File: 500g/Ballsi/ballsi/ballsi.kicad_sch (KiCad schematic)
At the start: 4 parts, among them J1 Conn_01x03, J2 Conn_01x03, J3 Conn_01x03

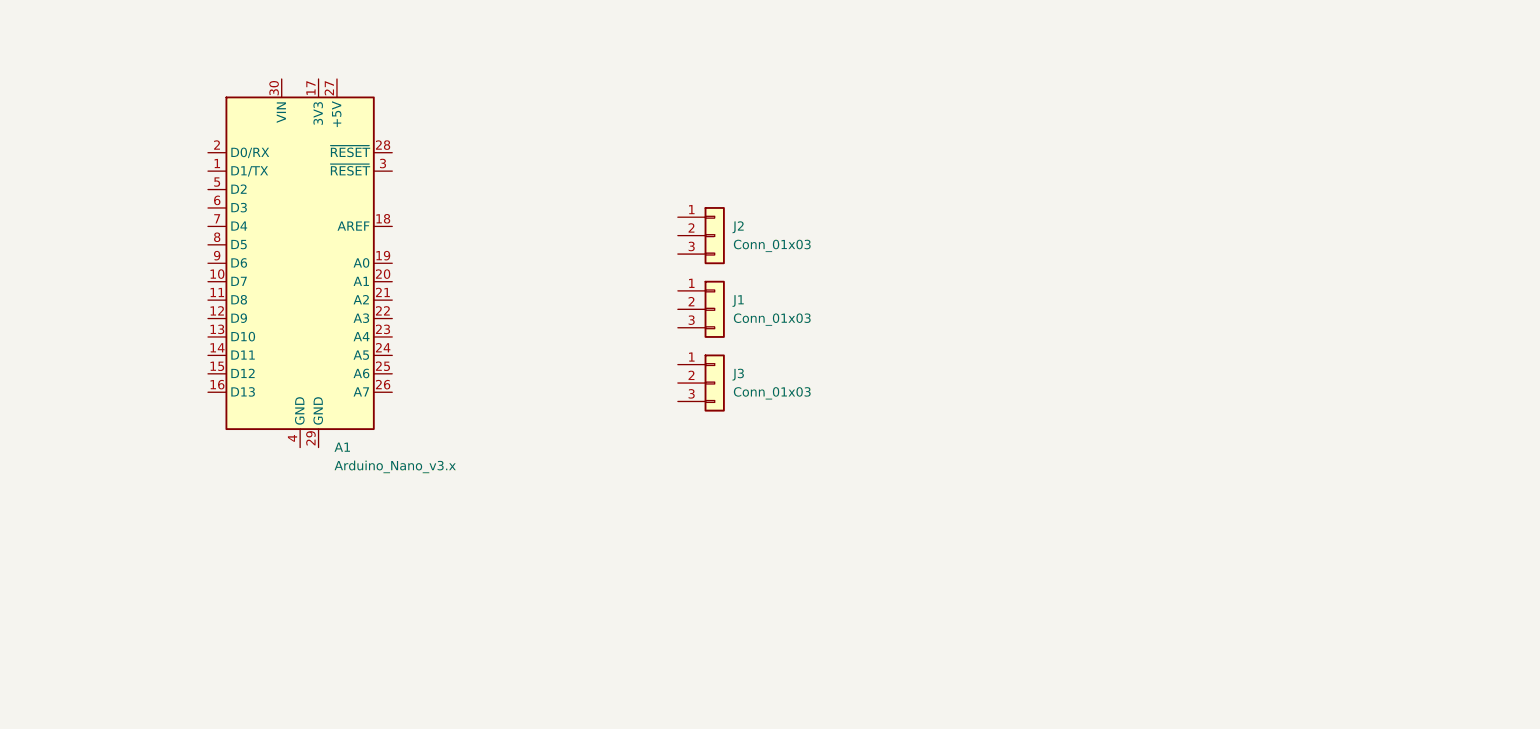
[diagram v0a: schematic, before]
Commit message: added microcontroller sensors and motordriver
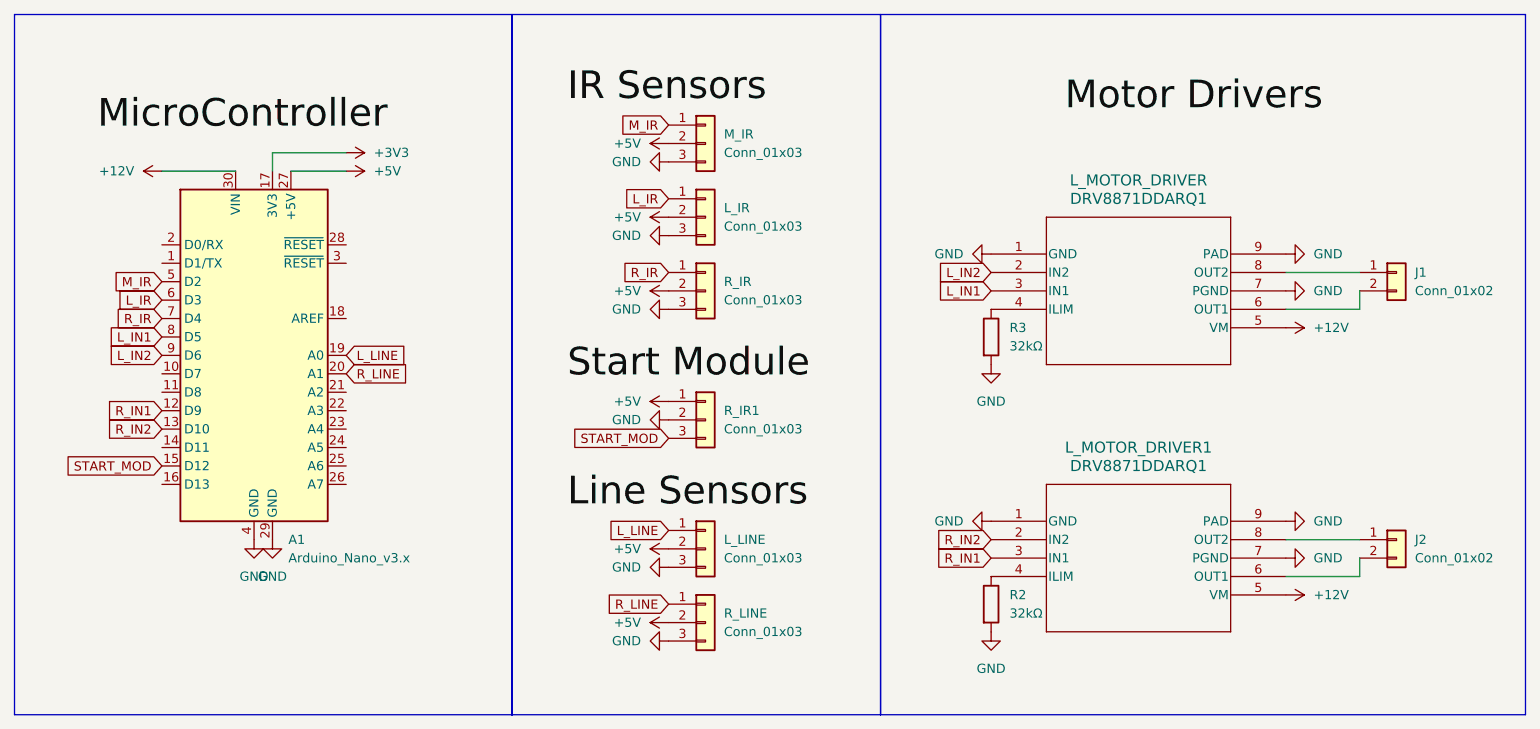
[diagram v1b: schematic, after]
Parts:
- added J1, J2: Conn_01x02, symbol Connector_Generic:Conn_01x02
- added L_LINE, R_IR1, R_LINE: Conn_01x03, Connector_JST:JST_PH_B3B-PH-K_1x03_P2.00mm_Vertical, symbol Connector_Generic:Conn_01x03
- added L_MOTOR_DRIVER, L_MOTOR_DRIVER1: DRV8871DDARQ1, DDA0008H_N_TEX, symbol DRV8871:DRV8871DDARQ1
- added R2, R3: 32kΩ, symbol Device:R
- renumbered J1 to L_IR, J2 to M_IR, J3 to R_IR
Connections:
- net R_IN1: now reaches A1.12 (D9)
- net R_IN1: now also L_MOTOR_DRIVER1.3 (IN1)
- net R_IN2: now reaches A1.13 (D10)
- net R_IN2: now also L_MOTOR_DRIVER1.2 (IN2)
- net START_MOD: now reaches A1.15 (D12)
- net START_MOD: now also R_IR1.3 (Pin_3)
- net +3V3: now reaches A1.17 (3V3)
- net L_LINE: now reaches A1.19 (A0)
- net L_LINE: now also L_LINE.1 (Pin_1)
- net R_LINE: now reaches A1.20 (A1)
- net R_LINE: now also R_LINE.1 (Pin_1)
- net +5V: now reaches A1.27 (+5V)
- net +5V: now also L_IR.2 (Pin_2), M_IR.2 (Pin_2), R_IR.2 (Pin_2), L_LINE.2 (Pin_2), R_IR1.1 (Pin_1), R_LINE.2 (Pin_2)
- net GND: now reaches A1.29 (GND)
- net GND: now also A1.4 (GND), L_IR.3 (Pin_3), M_IR.3 (Pin_3), R_IR.3 (Pin_3), L_LINE.3 (Pin_3), L_MOTOR_DRIVER.1 (GND), L_MOTOR_DRIVER.7 (PGND), L_MOTOR_DRIVER.9 (PAD), L_MOTOR_DRIVER1.1 (GND), L_MOTOR_DRIVER1.7 (PGND), L_MOTOR_DRIVER1.9 (PAD), R2.2, R3.2, R_IR1.2 (Pin_2), R_LINE.3 (Pin_3)
- net +12V: now reaches A1.30 (VIN)
- net +12V: now also L_MOTOR_DRIVER.5 (VM), L_MOTOR_DRIVER1.5 (VM)
- net M_IR: now reaches A1.5 (D2)
- net M_IR: now also M_IR.1 (Pin_1)
- net L_IR: now reaches A1.6 (D3)
- net L_IR: now also L_IR.1 (Pin_1)
- net R_IR: now reaches A1.7 (D4)
- net R_IR: now also R_IR.1 (Pin_1)
- net L_IN1: now reaches A1.8 (D5)
- net L_IN1: now also L_MOTOR_DRIVER.3 (IN1)
- net L_IN2: now reaches A1.9 (D6)
- net L_IN2: now also L_MOTOR_DRIVER.2 (IN2)
- new net: L_MOTOR_DRIVER1.4 (ILIM), R2.1
- new net: J2.2 (Pin_2), L_MOTOR_DRIVER1.6 (OUT1)
- new net: J2.1 (Pin_1), L_MOTOR_DRIVER1.8 (OUT2)
- new net: L_MOTOR_DRIVER.4 (ILIM), R3.1
- new net: J1.1 (Pin_1), L_MOTOR_DRIVER.8 (OUT2)
- new net: J1.2 (Pin_2), L_MOTOR_DRIVER.6 (OUT1)
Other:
- moved on the sheet: A1, L_IR, M_IR, R_IR
